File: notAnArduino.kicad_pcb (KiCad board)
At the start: 2 copper layers, 20 parts, among them J1 PORTC, J2 PORTD, J3 PORTB, J4 AVR_ISP, J5 DC_IN, SW1 SW_RST, U1 ATmega328P-AU, U2 LM1117-5.0, Y1 8MHz Crystal

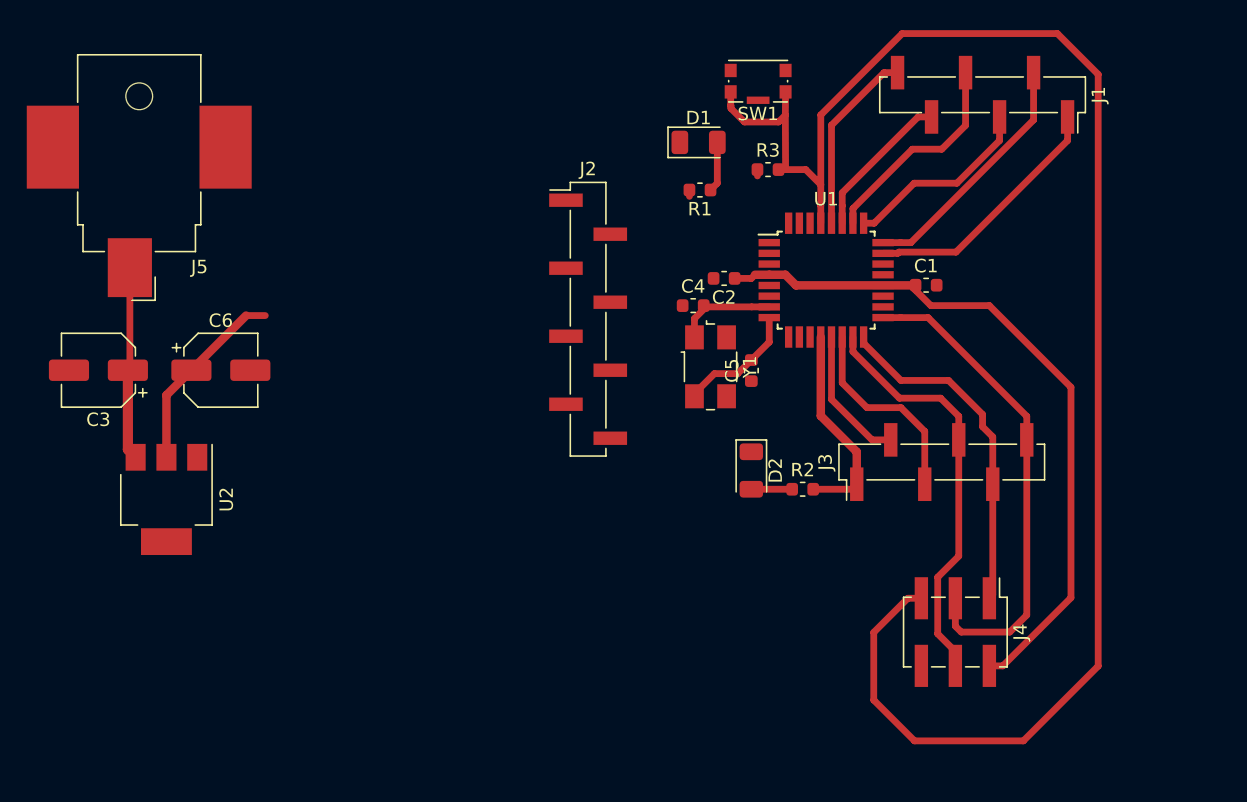
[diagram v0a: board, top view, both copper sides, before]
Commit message: foo
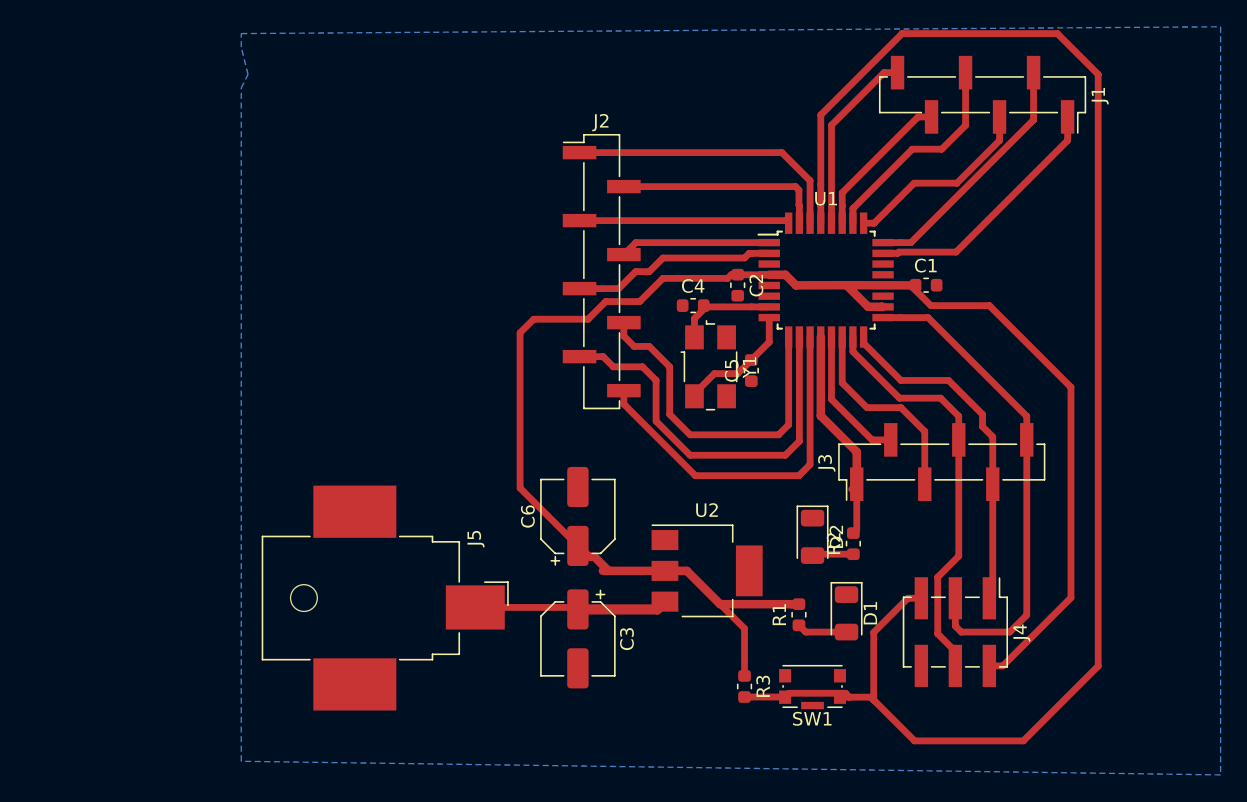
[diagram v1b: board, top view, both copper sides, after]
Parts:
- moved SW1 45.4 mm to (179.3, 94.5)
- moved C3 41.1 mm to (161.8, 90.9), turned to 270 degrees
- moved U2 40.7 mm to (171.4, 85.9), turned to 0 degrees
- moved R3 38.6 mm to (174.2, 94.5), turned to 270 degrees
- moved D1 36.9 mm to (181.9, 89.0), turned to 270 degrees
- moved J5 36.1 mm to (148.3, 87.9), turned to 270 degrees
- moved R1 32.6 mm to (178.3, 89.1), turned to 90 degrees
- moved C6 28.8 mm to (161.8, 81.8), turned to 90 degrees
- moved D2 6.74 mm to (179.3, 83.3)
- moved R2 5.55 mm to (182.4, 83.8), turned to 90 degrees
- moved J2 3.70 mm to (163.6, 63.5)
- moved C2 1.14 mm to (173.7, 64.5), turned to 270 degrees
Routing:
- net +5V: track 68.2 -> 116.9 mm
- net Net-(J2-Pad7): track 0.00 -> 29.5 mm
- net Net-(J2-Pad8): track 0.00 -> 27.0 mm
- net Net-(J2-Pad6): track 0.00 -> 25.3 mm
- net Net-(J2-Pad1): track 0.00 -> 21.3 mm
- net Net-(J2-Pad3): track 0.00 -> 15.7 mm
- net Net-(J2-Pad2): track 0.00 -> 15.7 mm
- net Net-(J2-Pad5): track 0.00 -> 15.3 mm
- net Net-(J2-Pad4): track 0.00 -> 11.2 mm
- net /NRST: track 122.6 -> 117.5 mm
- net /LED1: track 15.5 -> 16.4 mm
- added copper zone on B.Cu, net GND
